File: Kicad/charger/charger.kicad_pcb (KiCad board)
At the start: 2 copper layers, 78 x 57 mm, 21 parts, among them K1 Charger, K2 Battery, Q1 STN790A, U1 BQ2057W

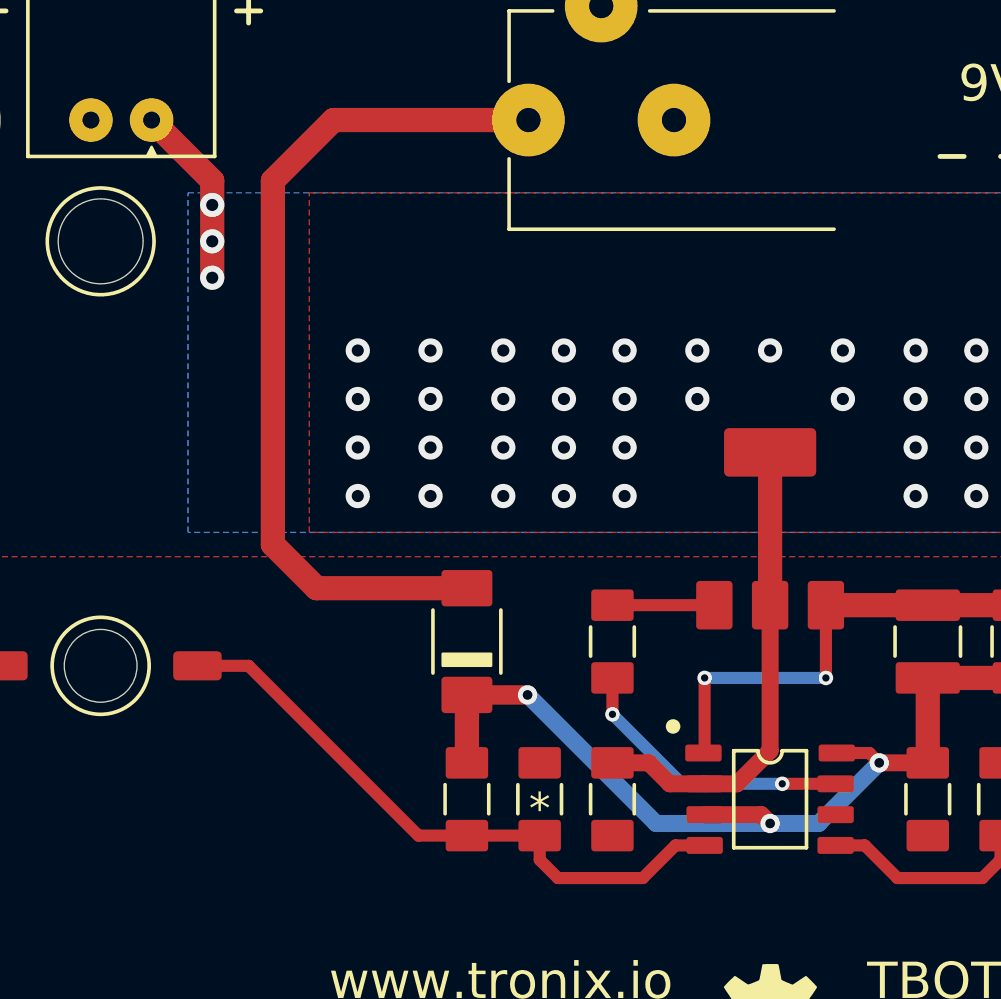
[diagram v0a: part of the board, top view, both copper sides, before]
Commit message: Update
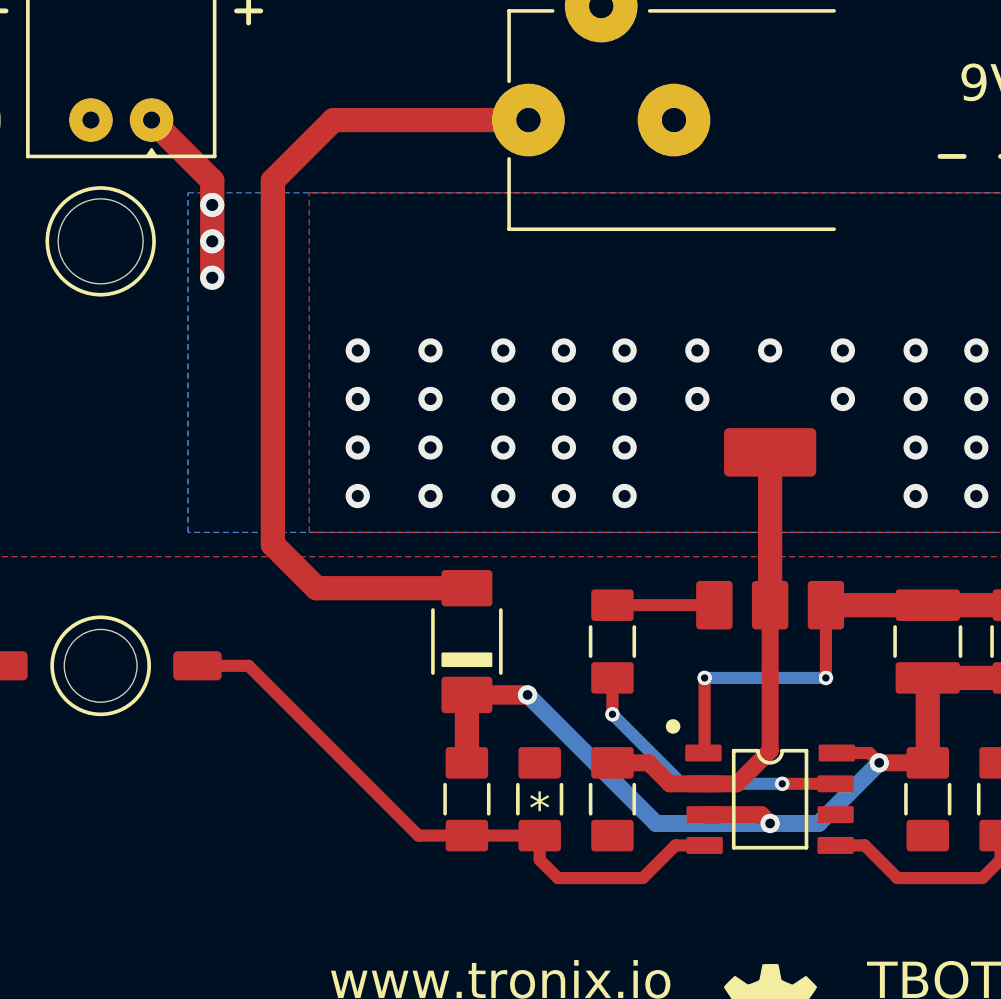
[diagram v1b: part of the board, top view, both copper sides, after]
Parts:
- C1, C2: footprint tronixio:CAPACITOR-1206 -> tronixio:CAPACITOR-SMD-1206
- H1, H2, H3: footprint tronixio:M3-MASK -> tronixio:MOUNTING-HOLE-3MM-MASK
- LED1: footprint tronixio:LED-1206 -> tronixio:LED-SMD-1206
- R1, R4, R5, R6: footprint tronixio:RESISTOR-1206 -> tronixio:RESISTOR-SMD-1206
- R2, R3: footprint tronixio:RESISTOR-1210 -> tronixio:RESISTOR-SMD-1210

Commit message: Update
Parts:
- K1: value Charger -> 9V - 1A
